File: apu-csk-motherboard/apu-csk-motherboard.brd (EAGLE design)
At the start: 90.2 x 95.9 mm, 27 parts, among them J2 TSW-108-05-G-S, P1 ATECC608A-SSHDA-B, T1 DS18B20, T2 DS18B20, T3 DS18B20, T4 DS18B20, U1 DS3231M+TRL

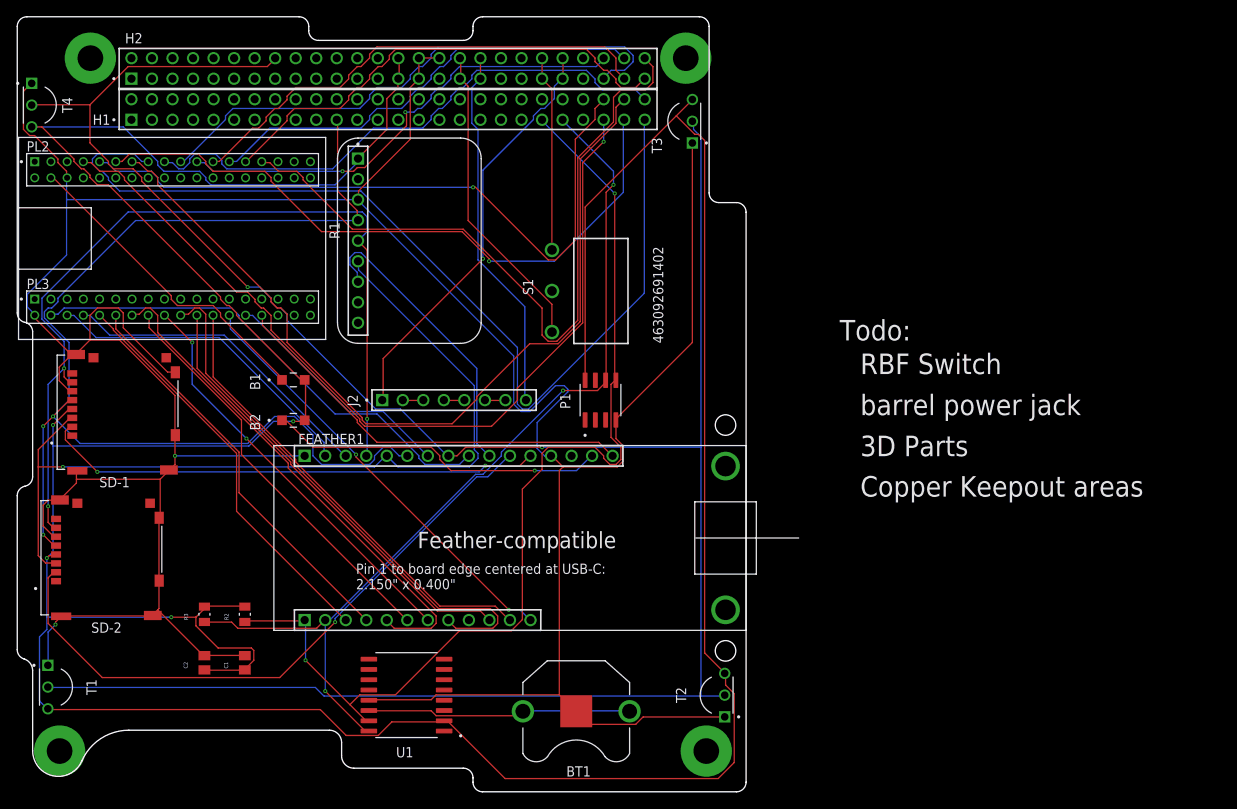
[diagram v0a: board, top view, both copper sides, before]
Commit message: JR to review
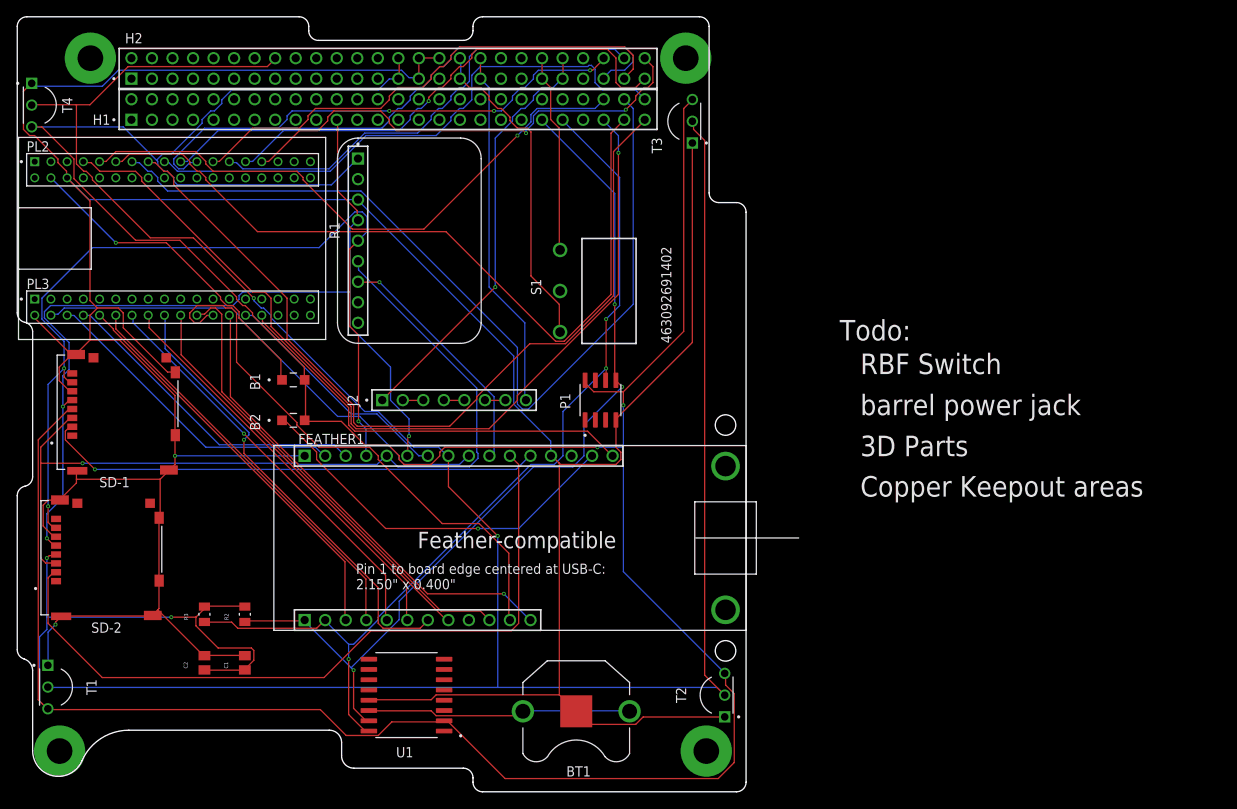
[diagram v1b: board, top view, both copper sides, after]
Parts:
- moved S1 1.00 mm to (67.0, 62.0)
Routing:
- net USER11: track 90.0 -> 59.7 mm, vias 0 -> 2
- net 3.3V: track 442.9 -> 470.9 mm
- net SCK: track 145.0 -> 118.8 mm
- net GND: track 420.2 -> 439.0 mm
- net SDA: track 128.8 -> 112.2 mm, vias 2 -> 3
- net FE_IO11: track 67.6 -> 51.7 mm
- net USER4: track 120.7 -> 106.1 mm
- net USER2: track 81.9 -> 96.3 mm, vias 1 -> 0
- net CS-SD-2: track 78.5 -> 91.9 mm, vias 1 -> 0
- net FE_IO2: track 63.1 -> 50.9 mm, vias 0 -> 1
- net FE_EN: track 57.0 -> 69.1 mm
- net USER1: track 84.1 -> 74.5 mm
- net CS-FRAM: track 36.8 -> 30.3 mm, vias 0 -> 1
- net UC3.3: track 42.0 -> 48.2 mm
- net FE_IO10: track 51.2 -> 56.4 mm, vias 2 -> 1
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
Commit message: RBF Placement
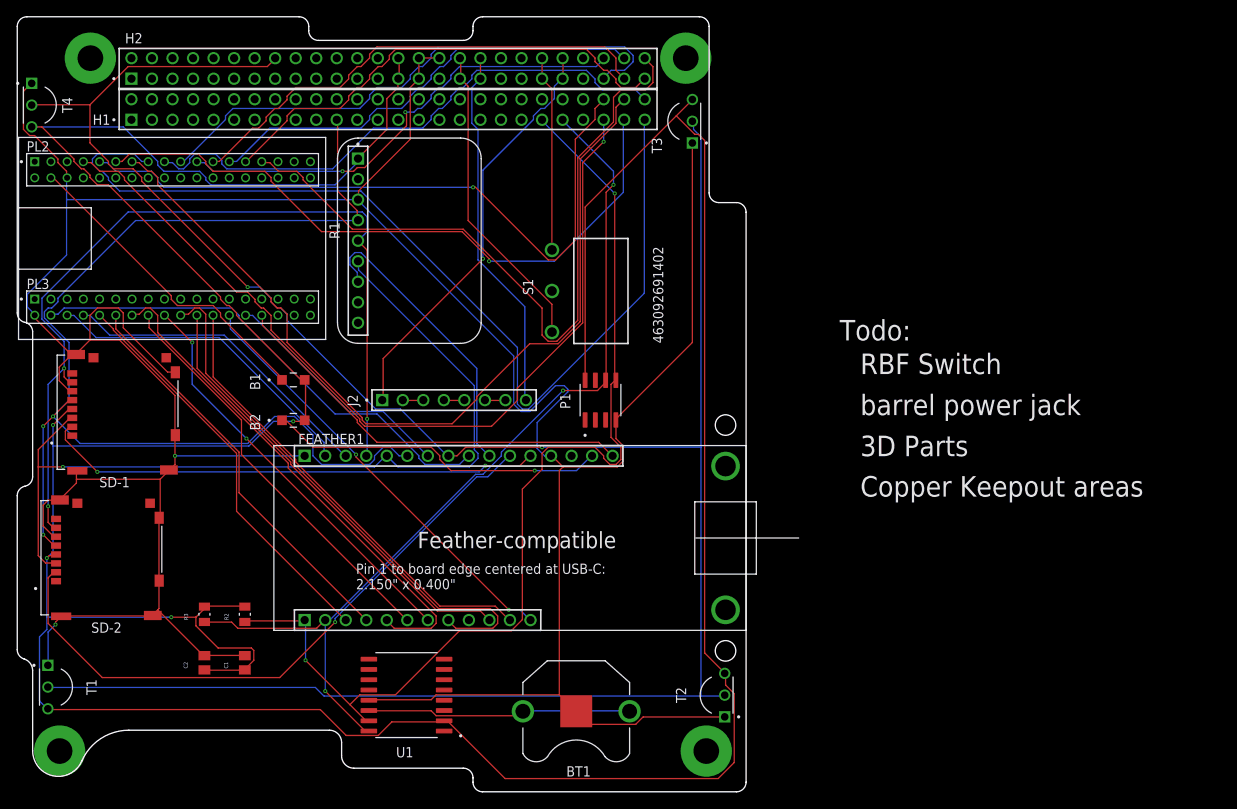
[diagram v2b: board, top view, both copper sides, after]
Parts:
- moved S1 1.00 mm to (66.0, 62.0)
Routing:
- net USER11: track 59.7 -> 90.0 mm, vias 2 -> 0
- net 3.3V: track 470.9 -> 442.9 mm
- net SCK: track 118.8 -> 145.0 mm
- net GND: track 439.0 -> 420.2 mm
- net SDA: track 112.2 -> 128.8 mm, vias 3 -> 2
- net FE_IO11: track 51.7 -> 67.6 mm
- net USER4: track 106.1 -> 120.7 mm
- net USER2: track 96.3 -> 81.9 mm, vias 0 -> 1
- net CS-SD-2: track 91.9 -> 78.5 mm, vias 0 -> 1
- net FE_IO2: track 50.9 -> 63.1 mm, vias 1 -> 0
- net FE_EN: track 69.1 -> 57.0 mm
- net USER1: track 74.5 -> 84.1 mm
- net CS-FRAM: track 30.3 -> 36.8 mm, vias 1 -> 0
- net UC3.3: track 48.2 -> 42.0 mm
- net FE_IO10: track 56.4 -> 51.2 mm, vias 1 -> 2
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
